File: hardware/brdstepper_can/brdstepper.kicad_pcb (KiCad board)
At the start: 4 copper layers, 28 x 28 mm, 89 parts, among them J1 USB-C, J2 VM / GND / EN, J3 MOTOR, J5 CAN, J6 CAN, J7 SWD, U1 STM32G473CEU6, U2 DRV8876RGTR, U3 DRV8876RGTR, U4 AS5047P-ATSM, U5 TLV75533PDBVR, U6 TPS560430XDBVR, U7 USBLC6-2SC6, U9 TCAN1044VDR, Y1 8MHz

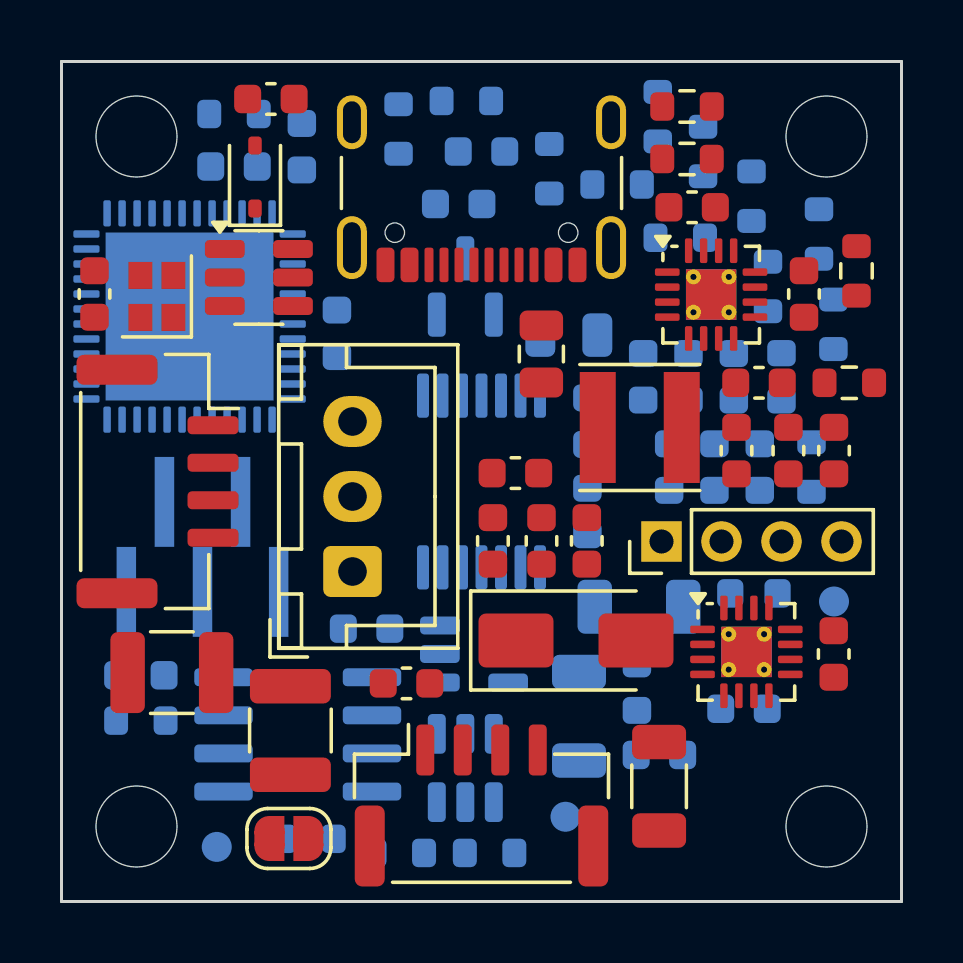
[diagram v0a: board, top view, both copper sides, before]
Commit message: brdstepper: re-placed boards without J2 (routing run in progress)
Both boards re-placed with J2 gone, courtyard gap 0.40 mm. Snapshot taken
while the first plane-aware routing run is still going: copper may be
missing or partial.

Co-Authored-By: Claude Sonnet 5.5 <noreply@anthropic.com>
Claude-Session: https://claude.ai/code/session_017CSpK2B8oMBAmr39Kq1RSC
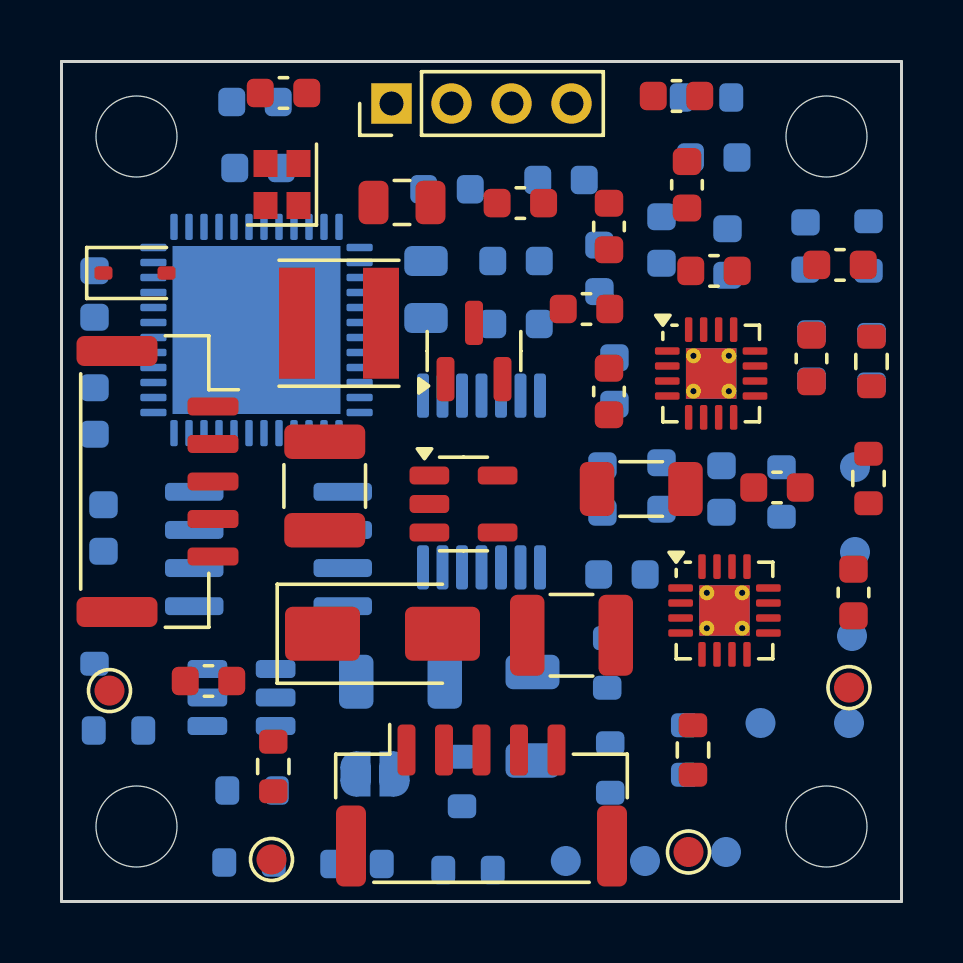
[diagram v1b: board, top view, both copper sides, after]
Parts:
- removed C37: 4.7n, Capacitor_SMD:C_0603_1608Metric
- removed J1: USB-C, Connector_USB:USB_C_Receptacle_GCT_USB4105-xx-A_16P_TopMnt_Horizontal
- removed J2: VM / GND / EN, Connector_JST:JST_XH_B3B-XH-A_1x03_P2.50mm_Vertical
- removed J7: SWD, Connector_PinHeader_1.27mm:PinHeader_1x05_P1.27mm_Vertical_SMD_Pin1Left
- removed R17, R18: 5.1k, Resistor_SMD:R_0603_1608Metric
- removed R19: 1M, Resistor_SMD:R_0603_1608Metric
- removed U7: USBLC6-2SC6, Package_TO_SOT_SMD:SOT-23-6
- added TP10: USB D+, TestPoint:TestPoint_Pad_D1.0mm, F.Cu at (87.6, 107.0)
- added TP11: USB D-, TestPoint:TestPoint_Pad_D1.0mm, F.Cu at (93.0, 112.6)
- added TP12: USB GND, TestPoint:TestPoint_Pad_D1.0mm, B.Cu at (112.5, 102.3)
- added TP4: SWD 3V3, TestPoint:TestPoint_Pad_D1.0mm, B.Cu at (112.5, 99.5)
- added TP5: SWDIO, TestPoint:TestPoint_Pad_D1.0mm, F.Cu at (112.2, 106.9)
- added TP6: NRST, TestPoint:TestPoint_Pad_D1.0mm, B.Cu at (108.2, 112.3)
- added TP7: SWCLK, TestPoint:TestPoint_Pad_D1.0mm, B.Cu at (112.3, 105.2)
- added TP8: SWD GND, TestPoint:TestPoint_Pad_D1.0mm, B.Cu at (112.2, 108.0)
- added TP9: USB 5V, TestPoint:TestPoint_Pad_D1.0mm, B.Cu at (105.5, 112.7)
- C11, C13, C18, C22, C27, C28, C39, C6, JP1, R12, R13, R8: moved to B.Cu
- C19, C21, C3, C30, C5, C7, C8, D1, R1, R14, R3, R7, TP2, U5: moved to F.Cu
- J5, J6: footprint Connector_JST:JST_GH_SM04B-GHS-TB_1x04-1MP_P1.25mm_Horizontal -> Connector_JST:JST_GH_SM05B-GHS-TB_1x05-1MP_P1.25mm_Horizontal
- moved R3 27.1 mm to (113.0, 96.0), turned to 90 degrees
- moved R4 25.6 mm to (112.9, 92.2), turned to 90 degrees
- moved R9 24.2 mm to (99.5, 113.0), turned to 0 degrees
- moved R16 24.1 mm to (92.3, 110.3)
- moved R2 22.9 mm to (92.2, 112.7), turned to 0 degrees
- moved R1 22.2 mm to (93.1, 109.5), turned to 90 degrees
- moved R15 22.1 mm to (87.9, 108.3), turned to 0 degrees
- moved R7 18.6 mm to (107.0, 109.0)
- moved R10 18.1 mm to (87.1, 105.2), turned to 90 degrees
- moved J3 17.2 mm to (97.0, 87.4)
- moved R8 17.0 mm to (106.8, 109.0)
- moved TH1 16.6 mm to (104.3, 109.5)
- moved TP2 15.7 mm to (106.9, 112.3)
- moved C5 15.2 mm to (90.9, 106.7)
- moved C19 15.1 mm to (101.3, 90.7)
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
